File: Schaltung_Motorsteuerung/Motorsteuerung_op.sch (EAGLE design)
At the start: 10 parts, among them IC1 ULN2003AN, IC2 LM324P

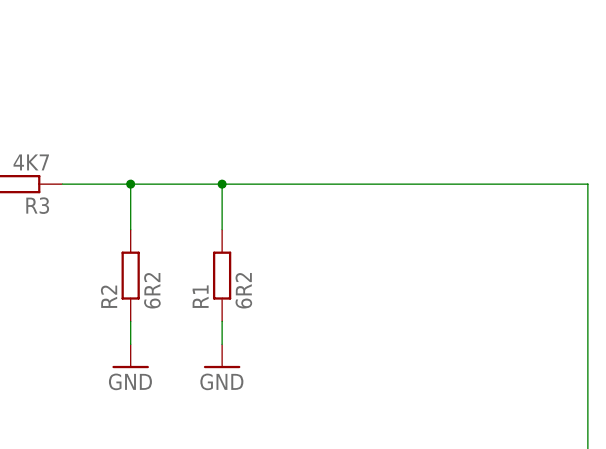
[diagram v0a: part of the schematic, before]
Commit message: Update 4
added more parts
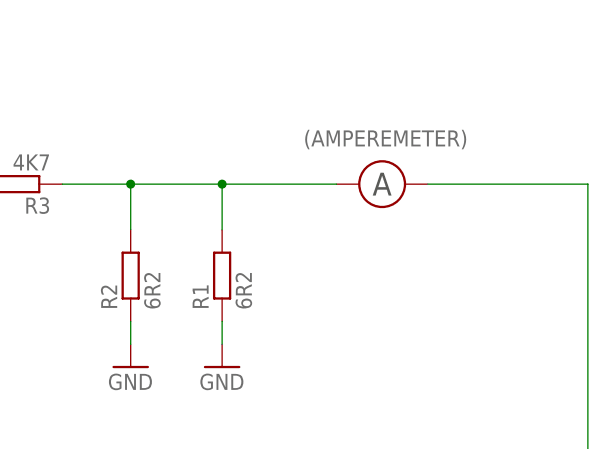
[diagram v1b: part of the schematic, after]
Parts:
- added (AMPEREMETER): MESSGERAET, luani_docuSymbol:MESSGERAET
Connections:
- new net N$10: (AMPEREMETER).P$2, R1.2, R2.2, R3.1
- net N$9: now also (AMPEREMETER).P$1; no longer R1.2, R2.2, R3.1
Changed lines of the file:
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@@
 <part name="GND7" library="supply1" library_urn="urn:adsk.eagle:library:371" deviceset="GND" device=""/>
 <part name="P+6" library="supply1" library_urn="urn:adsk.eagle:library:371" deviceset="VCC" device=""/>
+<part name="(AMPEREMETER)" library="luani_docuSymbol" deviceset="MESSGERAET" device="">
+<attribute name="TYP" value="A"/>
+</part>
 </parts>
 <sheets>
@@
 <attribute name="VALUE" x="73.66" y="134.62" size="1.778" layer="96" rot="R90"/>
 </instance>
+<instance part="(AMPEREMETER)" gate="G$1" x="137.16" y="121.92" smashed="yes" rot="R90">
+<attribute name="TYP" x="137.16" y="121.92" size="2.54" layer="97" rot="R180" align="center"/>
+<attribute name="NAME" x="146.685" y="127" size="1.778" layer="95" rot="R180" align="center-left"/>
+</instance>
 </instances>
 <busses>
@@
 <wire x1="86.36" y1="40.64" x2="160.02" y2="40.64" width="0.1524" layer="91"/>
 <wire x1="160.02" y1="40.64" x2="160.02" y2="121.92" width="0.1524" layer="91"/>
-<wire x1="160.02" y1="121.92" x2="119.38" y2="121.92" width="0.1524" layer="91"/>
-<pinref part="R3" gate="G$1" pin="1"/>
-<pinref part="R2" gate="G$1" pin="2"/>
-<wire x1="119.38" y1="121.92" x2="109.22" y2="121.92" width="0.1524" layer="91"/>
-<wire x1="109.22" y1="121.92" x2="101.6" y2="121.92" width="0.1524" layer="91"/>
-<wire x1="109.22" y1="116.84" x2="109.22" y2="121.92" width="0.1524" layer="91"/>
-<junction x="109.22" y="121.92"/>
-<pinref part="R1" gate="G$1" pin="2"/>
-<wire x1="119.38" y1="116.84" x2="119.38" y2="121.92" width="0.1524" layer="91"/>
-<junction x="119.38" y="121.92"/>
+<wire x1="160.02" y1="121.92" x2="142.24" y2="121.92" width="0.1524" layer="91"/>
+<pinref part="(AMPEREMETER)" gate="G$1" pin="P$1"/>
 </segment>
 </net>
@@
 </segment>
 </net>
+<net name="N$10" class="0">
+<segment>
+<pinref part="R3" gate="G$1" pin="1"/>
+<wire x1="109.22" y1="121.92" x2="101.6" y2="121.92" width="0.1524" layer="91"/>
+<pinref part="R2" gate="G$1" pin="2"/>
+<wire x1="109.22" y1="116.84" x2="109.22" y2="121.92" width="0.1524" layer="91"/>
+<junction x="109.22" y="121.92"/>
+<wire x1="119.38" y1="121.92" x2="109.22" y2="121.92" width="0.1524" layer="91"/>
+<pinref part="R1" gate="G$1" pin="2"/>
+<wire x1="119.38" y1="116.84" x2="119.38" y2="121.92" width="0.1524" layer="91"/>
+<junction x="119.38" y="121.92"/>
+<wire x1="132.08" y1="121.92" x2="119.38" y2="121.92" width="0.1524" layer="91"/>
+<pinref part="(AMPEREMETER)" gate="G$1" pin="P$2"/>
+</segment>
+</net>
